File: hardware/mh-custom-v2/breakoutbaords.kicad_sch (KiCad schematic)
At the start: 8 parts, among them J3 Conn_02x19_Top_Bottom, J4 Conn_02x19_Top_Bottom, U3 AMS1117-3.3

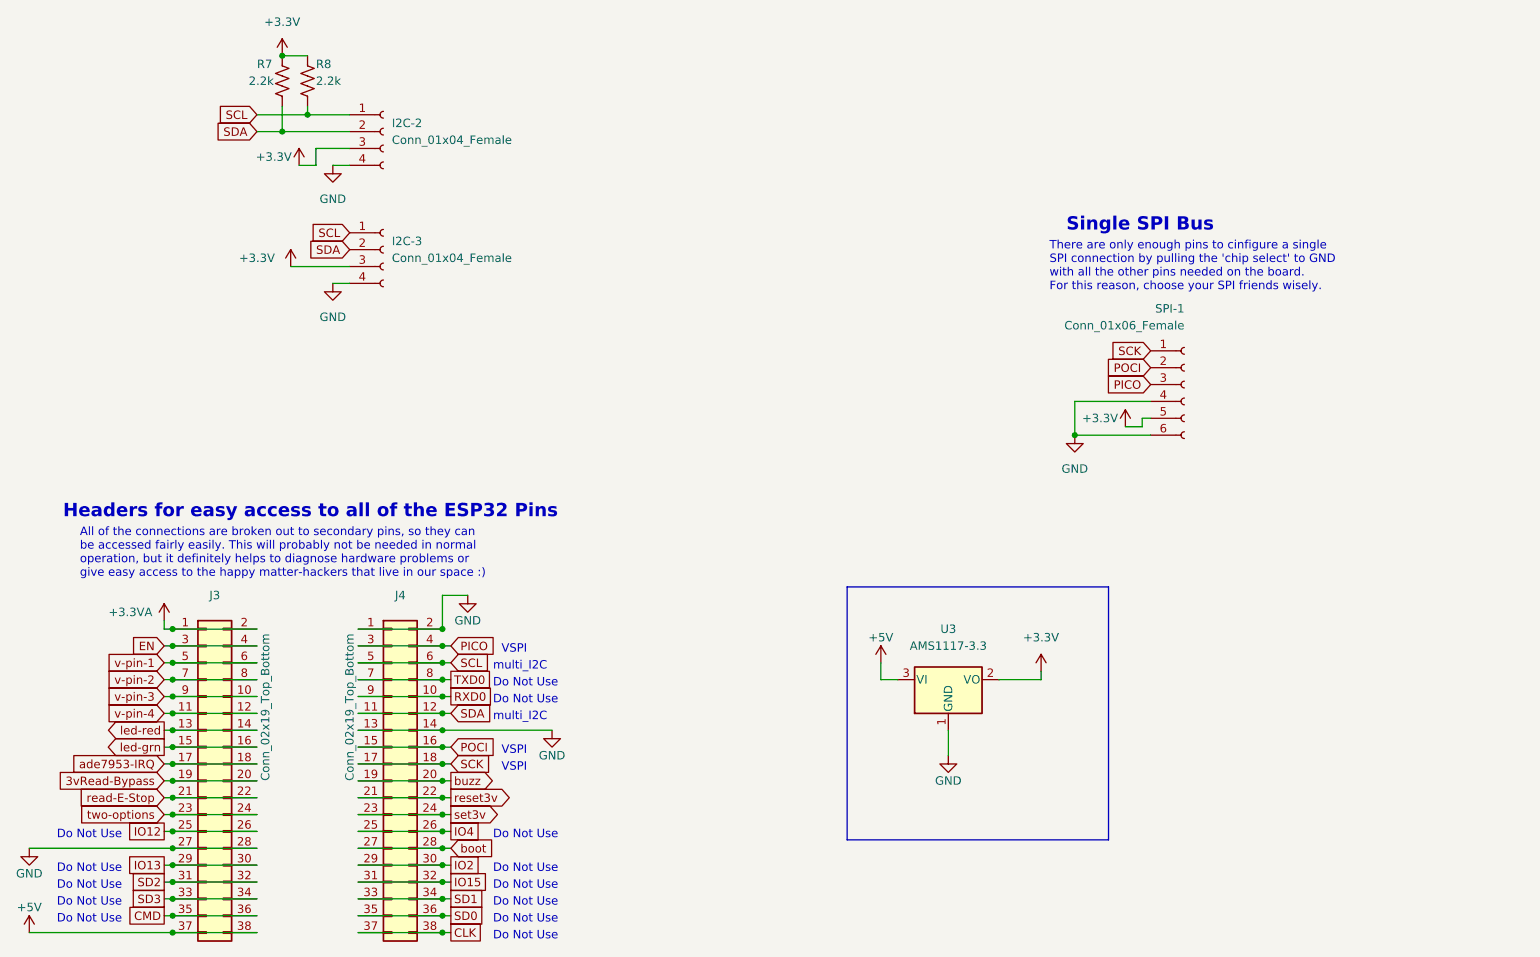
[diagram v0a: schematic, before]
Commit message: just ordered from JLCPCB
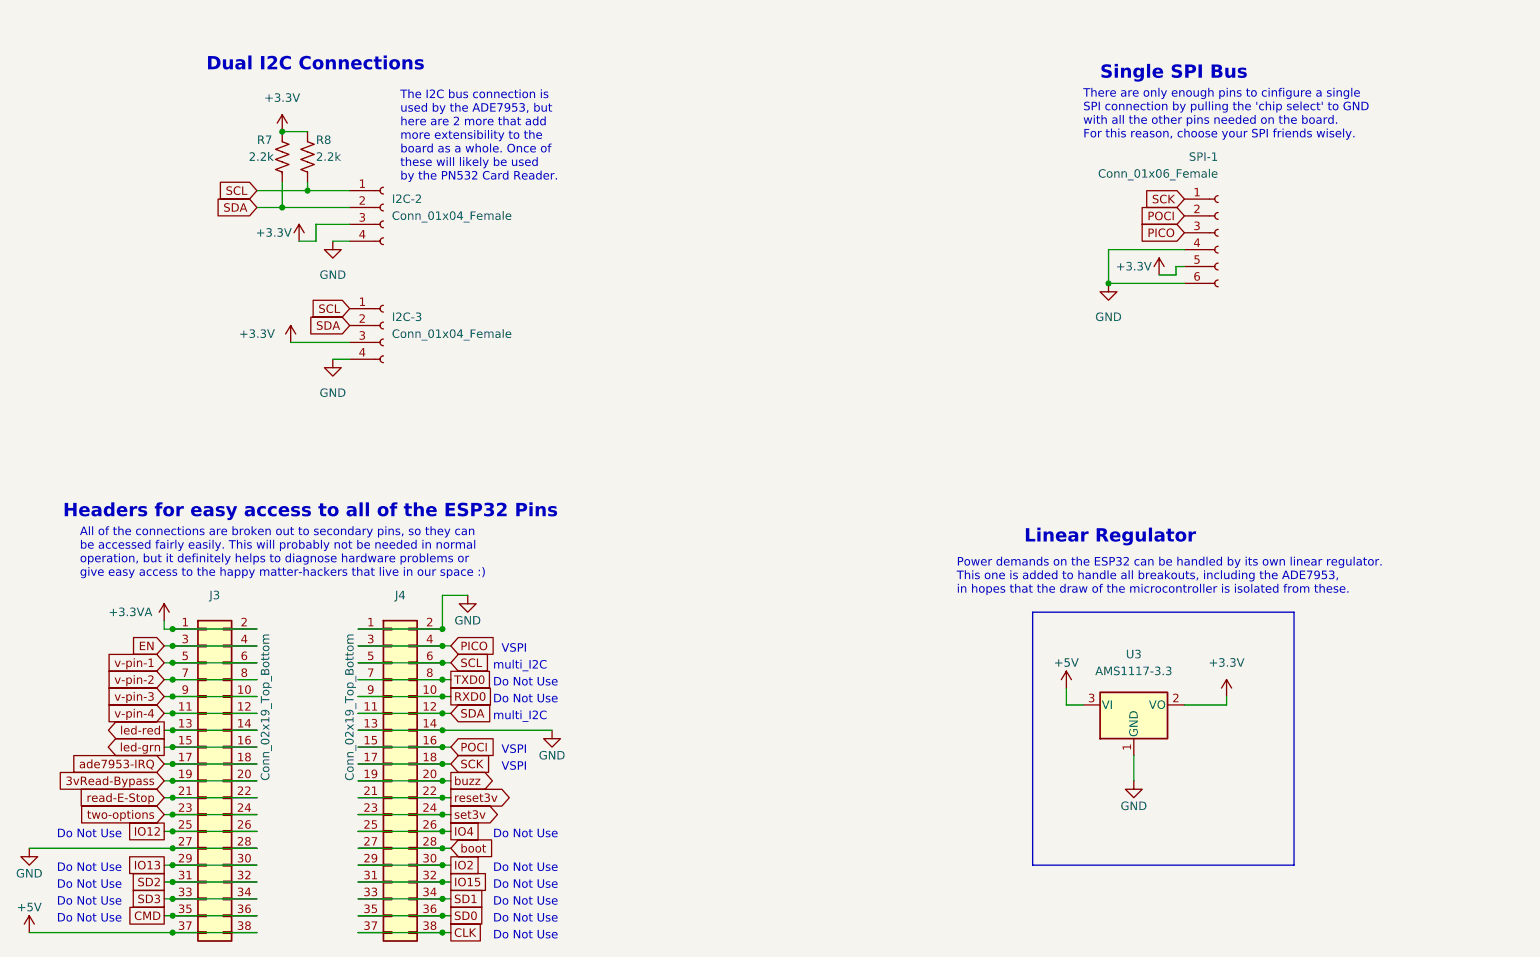
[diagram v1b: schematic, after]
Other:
- note added: "Dual I2C Connections"
- note added: "Linear Regulator"
- note added: "Power demands on the ESP32 can be handled by its own linear regulator. This one is added to handle all breakouts, including the ADE7953, in hopes that the draw of the microcontroller is isolated from these."
- note added: "The I2C bus connection is used by the ADE7953, but here are 2 more that add more extensibility to the board as a whole. Once of these will likely be used by the PN532 Card Reader."
- company: (none) -> Corey Rice & MakeHaven
- title: (none) -> Breakout Connections & Power
- moved on the sheet: I2C-2, I2C-3, R7, R8, SPI-1, U3
